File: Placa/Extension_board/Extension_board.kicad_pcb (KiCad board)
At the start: 2 copper layers, 61 x 20.3 mm, 12 parts, among them J1 Conn_01x05_Male, J2 USB_B_Micro, J3 Conn_01x04_Male, U1 STEVAL-STLCS01V1

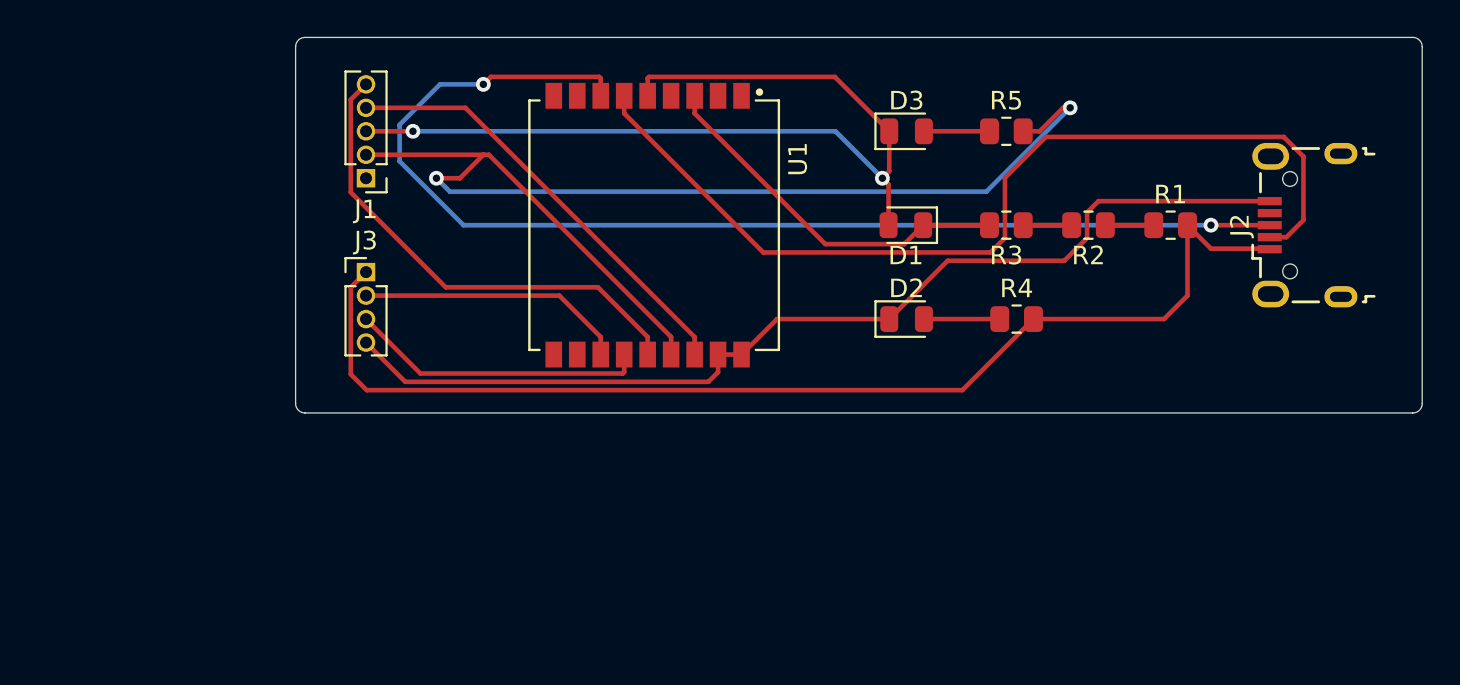
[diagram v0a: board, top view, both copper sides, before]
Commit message: Version 2.1 del proyecto
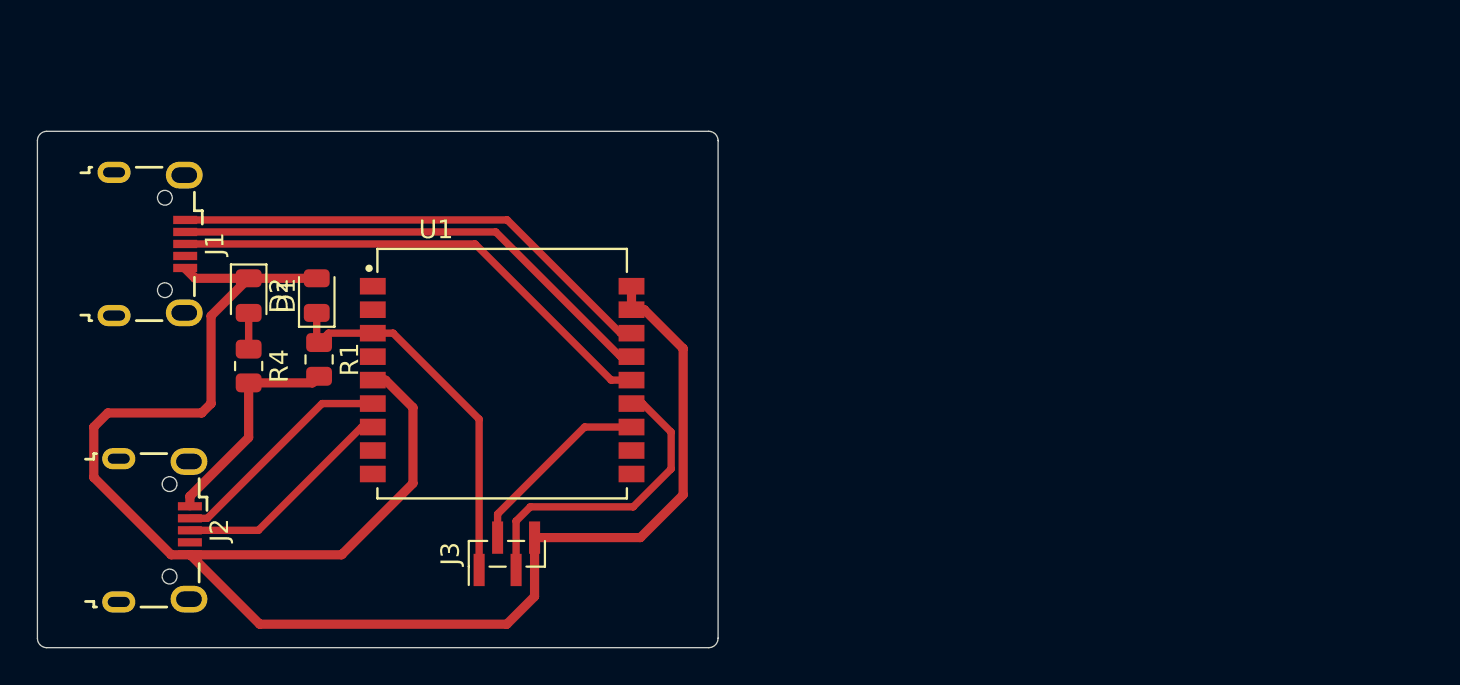
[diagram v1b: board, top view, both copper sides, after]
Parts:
- removed D3: LED, Diode_SMD:D_0805_2012Metric
- removed R2, R3: 1Ω, Resistor_SMD:R_0805_2012Metric
- removed R5: 1kΩ, Resistor_SMD:R_0805_2012Metric
- J1: value Conn_01x05_Male -> USB_B_Micro; footprint Connector_PinHeader_1.27mm:PinHeader_1x05_P1.27mm_Vertical -> Connector_USB:USB_Micro-B_Wuerth_629105150521
- J3: footprint Connector_PinHeader_1.27mm:PinHeader_1x04_P1.27mm_Vertical -> Connector_PinHeader_1.00mm:PinHeader_1x04_P1.00mm_Vertical_SMD_Pin1Left
- R1: value 1Ω -> 1,2Ω
- moved J2 64.4 mm to (102.9, 64.8), turned to 270 degrees
- moved R1 46.6 mm to (111.8, 55.5), turned to 270 degrees
- moved R4 41.6 mm to (108.0, 55.9), turned to 270 degrees
- moved D2 35.6 mm to (108.0, 52.1), turned to 270 degrees
- moved D1 32.1 mm to (111.6, 52.1), turned to 90 degrees
- moved J3 17.0 mm to (121.9, 66.0), turned to 90 degrees
- moved J1 12.2 mm to (102.6, 49.3), turned to 270 degrees
- moved U1 11.5 mm to (121.7, 56.6), turned to 0 degrees
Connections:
- J1 pad 1: Net-(J1-Pad1) -> /SWDIO
- J1 pad 3: /GND -> /RESET
- J1 pad 4: /SWDIO -> Net-(J1-Pad4)
- J1 pad 5: /RESET -> /GND
- J3 pad 1: /V_USB -> /VIN
- R1 pad 1: Net-(R1-Pad1) -> /VIN
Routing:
- net /RXD-USB_DM: track 63.4 -> 12.2 mm, vias 2 -> 0
- net /V_USB: track 62.4 -> 11.9 mm
- net /RXD-USB_DP: track 51.4 -> 12.5 mm
- net /SWDCLK: track 64.1 -> 26.9 mm, vias 2 -> 0
- net /GND: track 104.8 -> 97.9 mm, vias 2 -> 0
- net /I2C_SDA: track 14.6 -> 10.5 mm
- net Net-(D3-Pad2): track 3.55 -> 0.00 mm
- net /SWDIO: track 23.9 -> 26.7 mm
- net Net-(R1-Pad1): track 2.62 -> 0.00 mm
- net Net-(R2-Pad2): track 2.62 -> 0.00 mm
- net Net-(D2-Pad2): track 4.10 -> 1.96 mm
- net /I2C_SCL: track 16.2 -> 17.0 mm
- net /RESET: track 26.4 -> 27.2 mm
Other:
- board size 61 x 20.3 mm -> 36.8 x 27.9 mm
- net class Default: trace_width 0.25 -> 0.4
- net class Power added: clearance 0.2, trace_width 0.5, via_dia 0.8, via_drill 0.4
